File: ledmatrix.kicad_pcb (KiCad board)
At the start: 2 copper layers, 75.6 x 37.8 mm, 32 parts, among them J1 BUS_IN1, J2 BUS_IN2, J3 BUS_OUT1, J4 BUS_OUT2, Q1 PMV50XP, Q2 PMV50XP, Q3 PMV50XP, Q4 PMV50XP, Q5 PMV50XP, Q6 PMV50XP, Q7 PMV50XP, Q8 PMV50XP, U1 1588BS, U2 STP08DP05, U3 1588BS, U4 STP08DP05, U5 74HC138

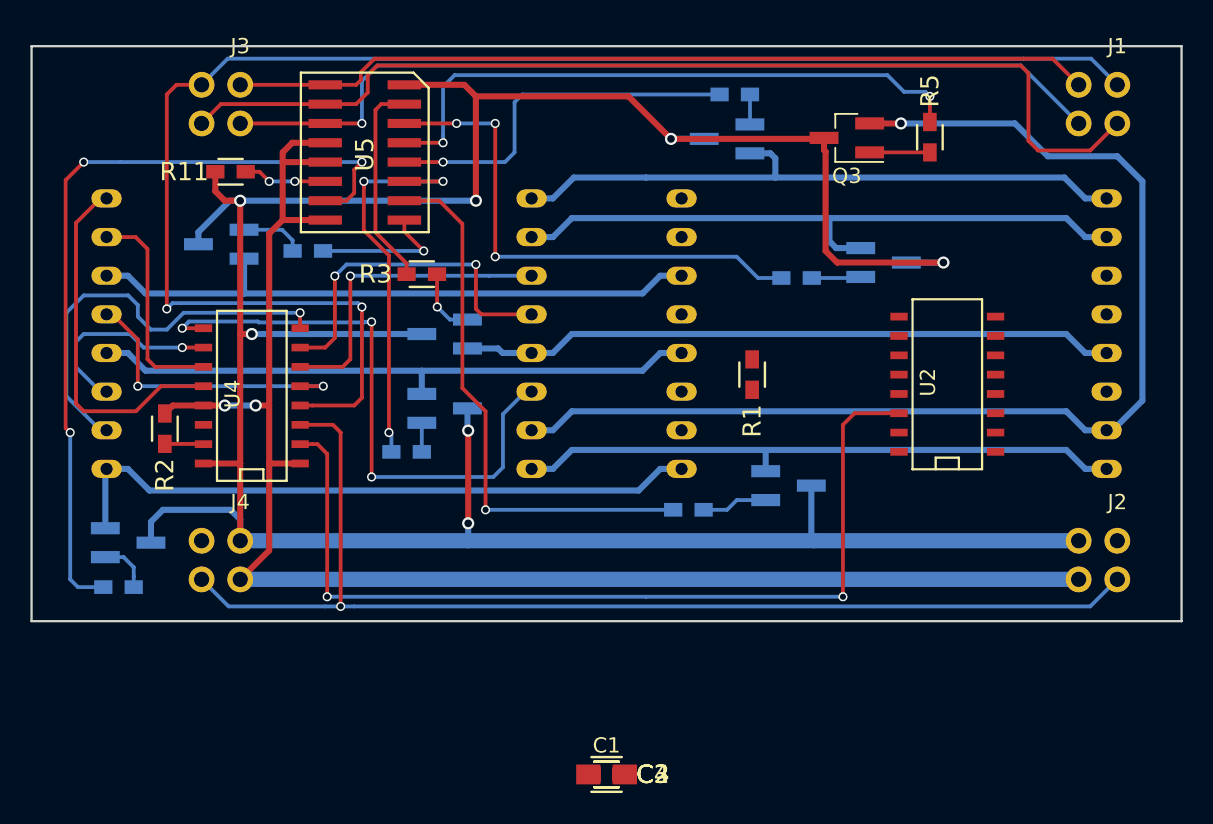
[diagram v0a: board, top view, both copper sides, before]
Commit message: fully connected PCB
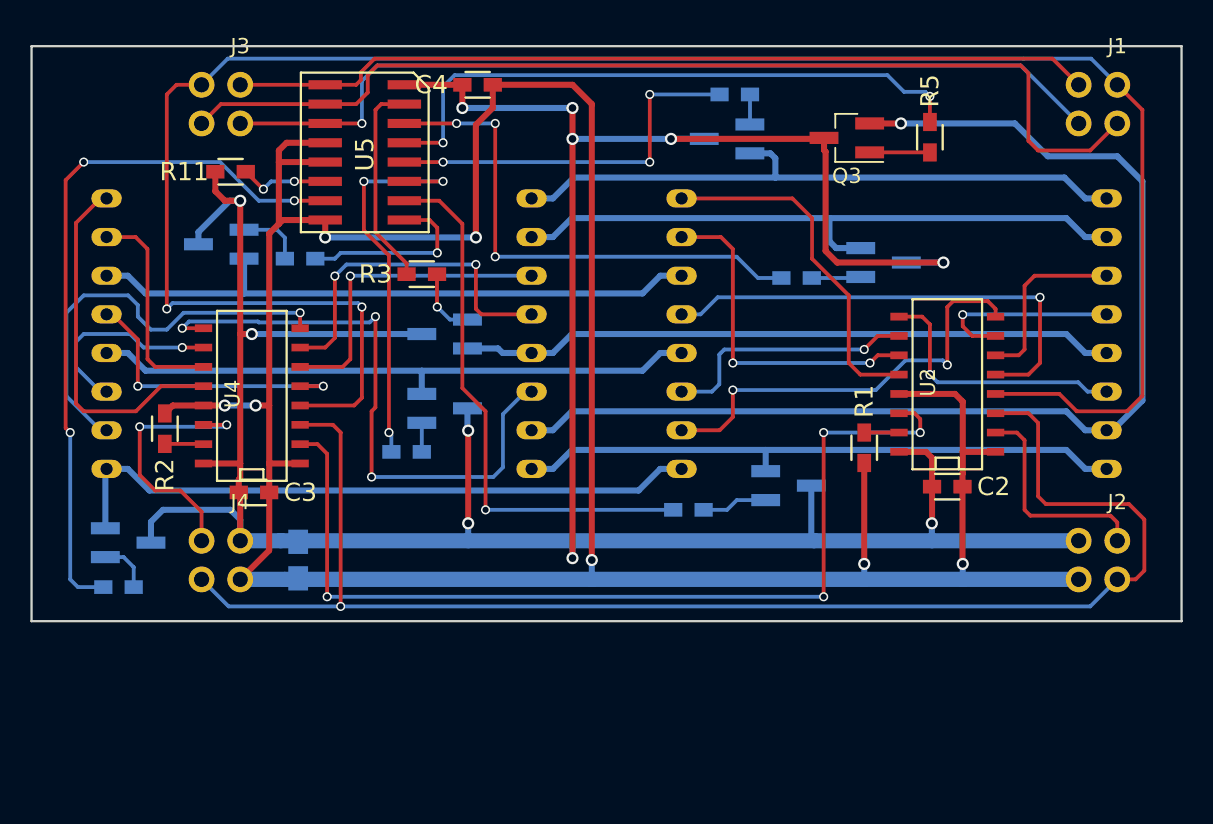
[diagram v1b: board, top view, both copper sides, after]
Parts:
- C1: moved to B.Cu
- moved C4 46.1 mm to (54.7, 27.9), turned to 180 degrees
- moved C3 29.7 mm to (40.0, 54.7)
- moved C2 29.3 mm to (85.6, 54.4)
- moved C1 24.7 mm to (42.9, 59.2), turned to 270 degrees
- moved R1 8.80 mm to (80.1, 51.8), turned to 90 degrees
- moved R9 0.72 mm to (43.1, 39.4)
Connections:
- C1 pad 1: (no net) -> /VCC
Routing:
- net /GND: track 102.1 -> 189.6 mm, vias 2 -> 7
- net /CLE: track 101.6 -> 133.3 mm
- net Net-(U1-Pad13): track 0.00 -> 31.6 mm, vias 0 -> 1
- net Net-(U1-Pad10): track 0.00 -> 28.4 mm, vias 0 -> 2
- net Net-(U1-Pad16): track 0.00 -> 23.3 mm
- net Net-(U1-Pad15): track 0.00 -> 22.3 mm, vias 0 -> 2
- net /CCK: track 76.3 -> 97.2 mm
- net /VCC: track 192.6 -> 210.4 mm, vias 7 -> 11
- net Net-(U1-Pad6): track 0.00 -> 17.6 mm, vias 0 -> 1
- net /CDO: track 0.00 -> 17.4 mm, vias 0 -> 2
- net Net-(U1-Pad11): track 0.00 -> 17.0 mm, vias 0 -> 1
- net /CDI: track 0.00 -> 14.3 mm
- net Net-(U1-Pad4): track 0.00 -> 12.6 mm, vias 0 -> 1
- net Net-(U1-Pad3): track 0.00 -> 11.9 mm
- net /Row Control/RC8: track 53.1 -> 48.2 mm
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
